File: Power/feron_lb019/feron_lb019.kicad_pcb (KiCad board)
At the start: 2 copper layers, 198 x 53 mm, 52 parts, among them J1 Conn_4pin01, J2 Conn_3pin01, P1 PC817, T1 TF8N60, U2 TL431, U3 OB2268

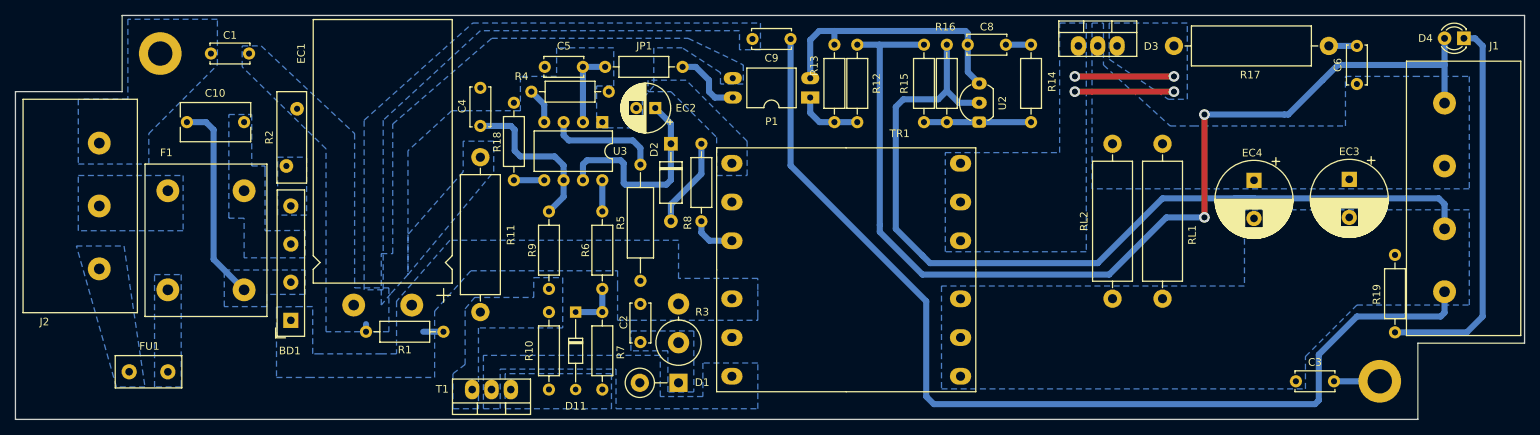
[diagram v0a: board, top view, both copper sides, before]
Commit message: Add L1R20C7
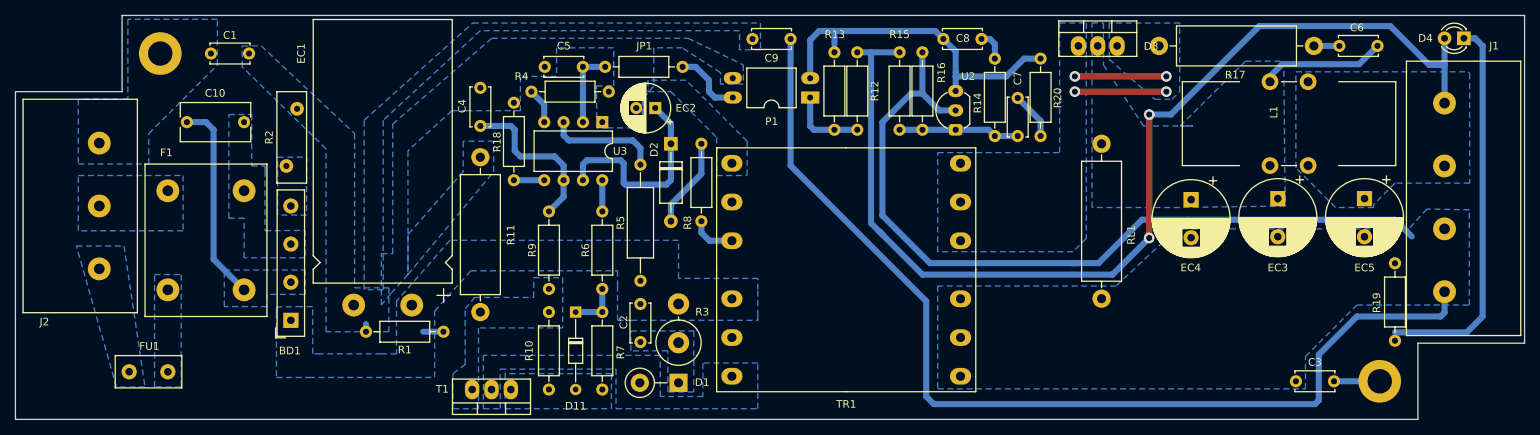
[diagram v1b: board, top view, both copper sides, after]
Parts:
- removed RL2: 2k, Resistor_THT:R_Axial_DIN0516_L15.5mm_D5.0mm_P20.32mm_Horizontal
- added C7: NA, Capacitor_THT:C_Disc_D5.0mm_W2.5mm_P5.00mm, F.Cu at (167.5, 85.8)
- added EC5: 1000x35, Capacitor_THT:CP_Radial_D10.0mm_P5.00mm, F.Cu at (213.0, 94.0)
- added L1: LFERR, _aTransformers:dross03, F.Cu at (208.1, 89.7)
- added R20: NA, Resistor_THT:R_Axial_DIN0207_L6.3mm_D2.5mm_P10.16mm_Horizontal, F.Cu at (170.5, 85.8)
- R15: value 33k -> 27k
- R16: value 3k -> 3k3
- moved EC3 9.71 mm to (201.6, 94.0)
- moved EC4 8.63 mm to (190.2, 94.2)
- moved RL1 8.00 mm to (178.5, 107.2)
- moved C6 5.68 mm to (214.7, 74.0), turned to 180 degrees
- moved R14 5.09 mm to (164.5, 85.8)
- moved R15 3.35 mm to (152.0, 85.0)
- moved R16 3.35 mm to (155.0, 74.8)
- moved C8 3.29 mm to (162.8, 73.1)
- moved U2 3.25 mm to (159.4, 85.0)
- moved R17 1.96 mm to (186.0, 74.0)
- moved R19 1.10 mm to (217.0, 102.5)
- moved R12 1.00 mm to (146.4, 85.0)
- moved R13 1.00 mm to (143.4, 74.8)
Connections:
- C6 pad 1: /+24V -> Net-(D3-K)
- D3 pad 2: /+24V -> Net-(D3-K)
- EC3 pad 1: /+24V -> Net-(D3-K)
- EC4 pad 1: /+24V -> Net-(D3-K)
- RL1 pad 2: /+24V -> Net-(D3-K)
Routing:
- net Net-(D3-K): track 0.00 -> 16.5 mm
- net GND: track 251.9 -> 239.9 mm
- net Net-(P1A-C): track 35.4 -> 45.3 mm
- net Net-(C7-Pad2): track 0.00 -> 6.24 mm
- net /+24V: track 137.5 -> 140.1 mm
- net Net-(D3-A1): track 26.0 -> 24.0 mm
- net Net-(U2-REF): track 14.0 -> 15.8 mm
- net Net-(P1A-A): track 8.68 -> 10.1 mm
- net Net-(C8-Pad1): track 3.25 -> 3.94 mm
- added copper zone on B.Cu, net Net-(D3-K)
